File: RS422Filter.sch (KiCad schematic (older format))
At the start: 13 parts, among them J12 Conn_01x02

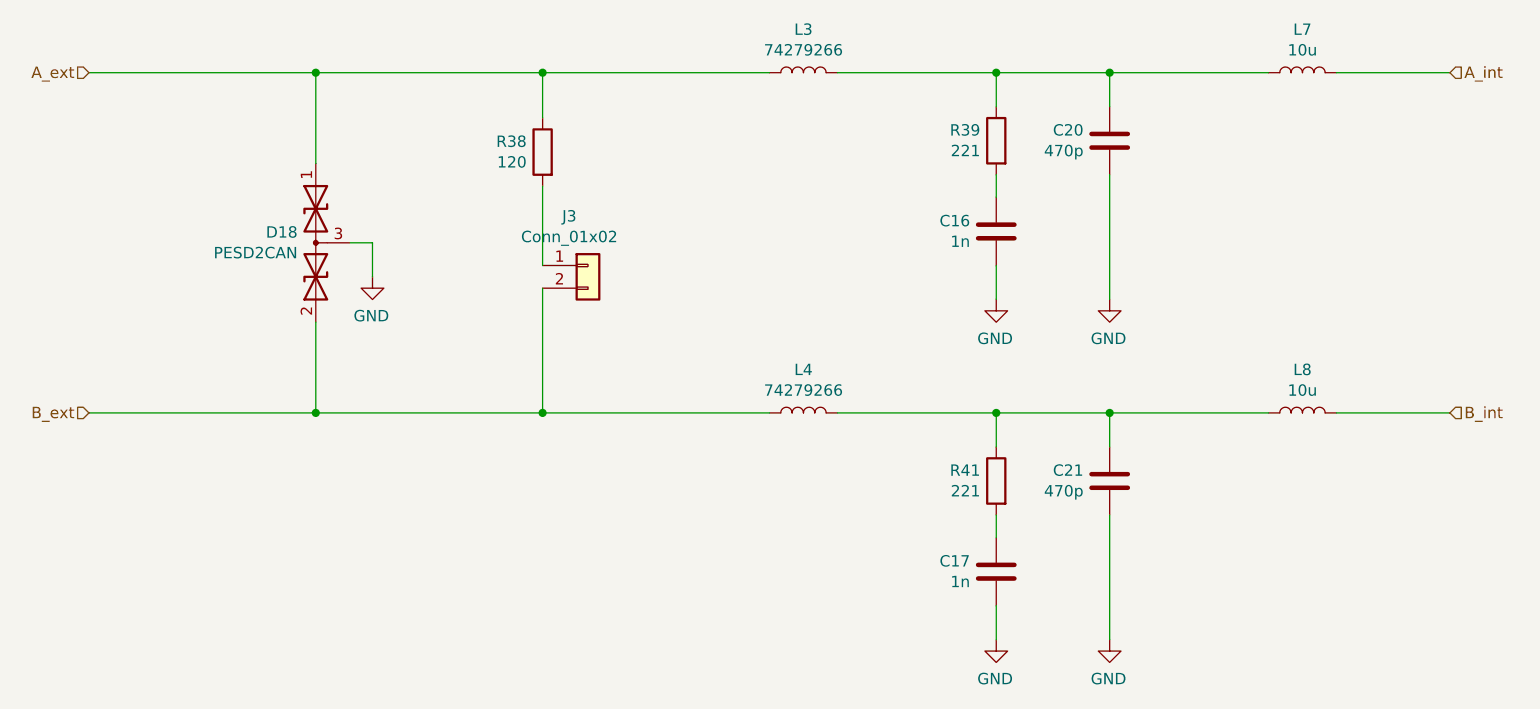
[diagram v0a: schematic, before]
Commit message: routing
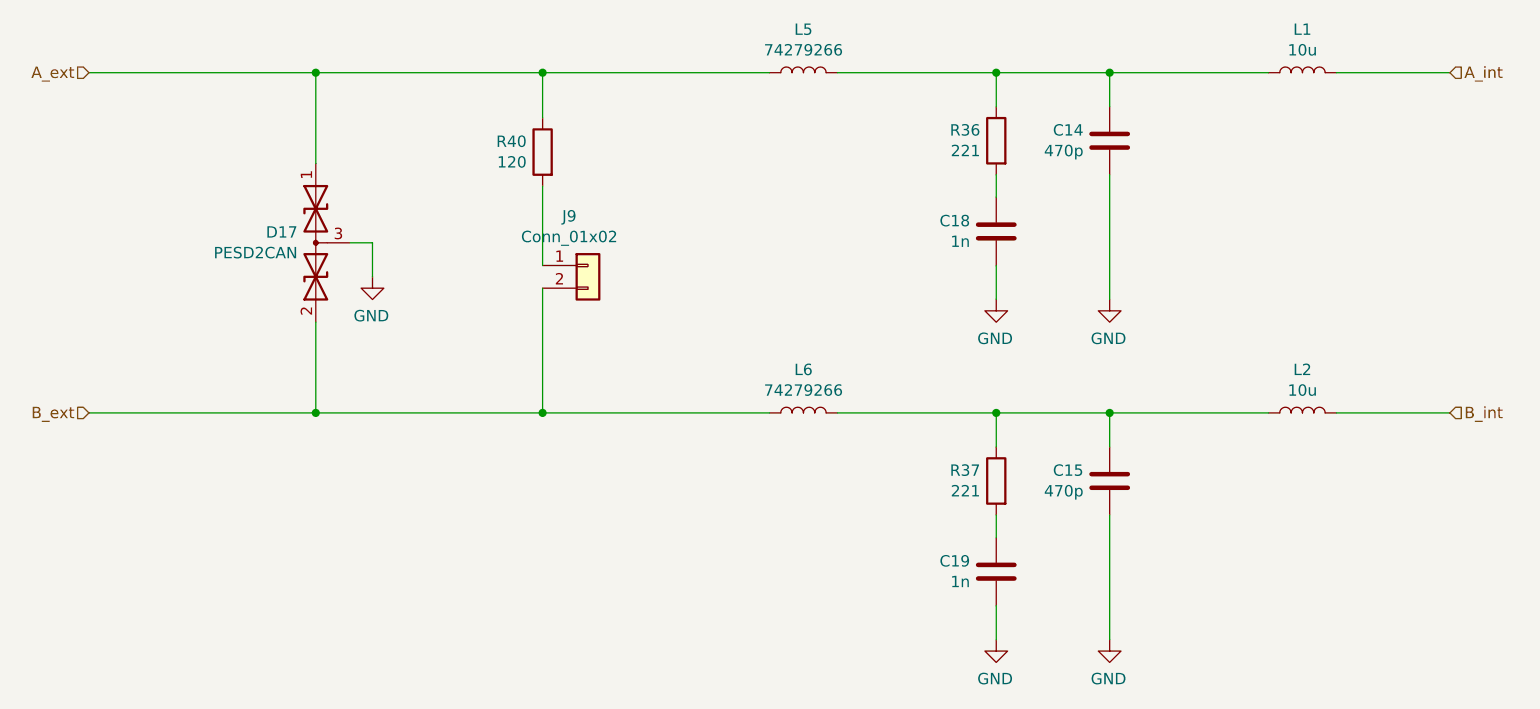
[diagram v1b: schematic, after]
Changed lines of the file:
@@
 $Descr A4 11693 8268
 encoding utf-8
-Sheet 5 22
+Sheet 4 22
 Title ""
 Date ""
@@
 AR Path="/6089ADE2/608D0C52/608D8603" Ref="D?"  Part="1"
 AR Path="/6089ADE2/608DD62D/608D8603" Ref="D18"  Part="1"
-F 0 "D18" V 3404 3330 50  0000 L CNN
+F 0 "D17" V 3404 3330 50  0000 L CNN
 F 1 "PESD2CAN" V 3495 3330 50  0000 L CNN
 F 2 "Package_TO_SOT_SMD:SOT-23_Handsoldering" H 3300 3250 50  0001 C CNN
@@
 AR Path="/6089ADE2/608D0C52/608D8609" Ref="L?"  Part="1"
 AR Path="/6089ADE2/608DD62D/608D8609" Ref="L3"  Part="1"
-F 0 "L3" V 5790 2500 50  0000 C CNN
+F 0 "L5" V 5790 2500 50  0000 C CNN
 F 1 "74279266" V 5699 2500 50  0000 C CNN
 F 2 "Inductor_SMD:L_0603_1608Metric" H 5600 2500 50  0001 C CNN
@@
 AR Path="/6089ADE2/608D0C52/608D985F" Ref="R?"  Part="1"
 AR Path="/6089ADE2/608DD62D/608D985F" Ref="R39"  Part="1"
-F 0 "R39" H 6520 2846 50  0000 L CNN
+F 0 "R36" H 6520 2846 50  0000 L CNN
 F 1 "221" H 6520 2755 50  0000 L CNN
 F 2 "Resistor_SMD:R_0603_1608Metric" V 6380 2800 50  0001 C CNN
@@
 AR Path="/6089ADE2/608D0C52/608D9BE8" Ref="C?"  Part="1"
 AR Path="/6089ADE2/608DD62D/608D9BE8" Ref="C16"  Part="1"
-F 0 "C16" H 6565 3246 50  0000 L CNN
+F 0 "C18" H 6565 3246 50  0000 L CNN
 F 1 "1n" H 6565 3155 50  0000 L CNN
 F 2 "Capacitor_SMD:C_0603_1608Metric" H 6488 3050 50  0001 C CNN
@@
 AR Path="/6089ADE2/608D0C52/608DA048" Ref="C?"  Part="1"
 AR Path="/6089ADE2/608DD62D/608DA048" Ref="C20"  Part="1"
-F 0 "C20" H 7065 2846 50  0000 L CNN
+F 0 "C14" H 7065 2846 50  0000 L CNN
 F 1 "470p" H 7065 2755 50  0000 L CNN
 F 2 "Capacitor_SMD:C_0603_1608Metric" H 6988 2650 50  0001 C CNN
@@
 AR Path="/6089ADE2/608D0C52/608DA55F" Ref="L?"  Part="1"
 AR Path="/6089ADE2/608DD62D/608DA55F" Ref="L7"  Part="1"
-F 0 "L7" V 7990 2500 50  0000 C CNN
+F 0 "L1" V 7990 2500 50  0000 C CNN
 F 1 "10u" V 7899 2500 50  0000 C CNN
 F 2 "Inductor_SMD:L_0603_1608Metric" H 7800 2500 50  0001 C CNN
@@
 AR Path="/6089ADE2/608D0C52/608DBE73" Ref="#PWR?"  Part="1"
 AR Path="/6089ADE2/608DD62D/608DBE73" Ref="#PWR0203"  Part="1"
-F 0 "#PWR0203" H 6450 3250 50  0001 C CNN
+F 0 "#PWR047" H 6450 3250 50  0001 C CNN
 F 1 "GND" H 6455 3327 50  0000 C CNN
 F 2 "" H 6450 3500 50  0001 C CNN
@@
 AR Path="/6089ADE2/608D0C52/608DC4B4" Ref="#PWR?"  Part="1"
 AR Path="/6089ADE2/608DD62D/608DC4B4" Ref="#PWR0204"  Part="1"
-F 0 "#PWR0204" H 6950 3250 50  0001 C CNN
+F 0 "#PWR043" H 6950 3250 50  0001 C CNN
 F 1 "GND" H 6955 3327 50  0000 C CNN
 F 2 "" H 6950 3500 50  0001 C CNN
@@
 AR Path="/6089ADE2/608D0C52/608E2FA4" Ref="L?"  Part="1"
 AR Path="/6089ADE2/608DD62D/608E2FA4" Ref="L4"  Part="1"
-F 0 "L4" V 5790 4000 50  0000 C CNN
+F 0 "L6" V 5790 4000 50  0000 C CNN
 F 1 "74279266" V 5699 4000 50  0000 C CNN
 F 2 "Inductor_SMD:L_0603_1608Metric" H 5600 4000 50  0001 C CNN
@@
 AR Path="/6089ADE2/608D0C52/608E2FAA" Ref="R?"  Part="1"
 AR Path="/6089ADE2/608DD62D/608E2FAA" Ref="R41"  Part="1"
-F 0 "R41" H 6520 4346 50  0000 L CNN
+F 0 "R37" H 6520 4346 50  0000 L CNN
 F 1 "221" H 6520 4255 50  0000 L CNN
 F 2 "Resistor_SMD:R_0603_1608Metric" V 6380 4300 50  0001 C CNN
@@
 AR Path="/6089ADE2/608D0C52/608E2FB0" Ref="C?"  Part="1"
 AR Path="/6089ADE2/608DD62D/608E2FB0" Ref="C17"  Part="1"
-F 0 "C17" H 6565 4746 50  0000 L CNN
+F 0 "C19" H 6565 4746 50  0000 L CNN
 F 1 "1n" H 6565 4655 50  0000 L CNN
 F 2 "Capacitor_SMD:C_0603_1608Metric" H 6488 4550 50  0001 C CNN
@@
 AR Path="/6089ADE2/608D0C52/608E2FB6" Ref="C?"  Part="1"
 AR Path="/6089ADE2/608DD62D/608E2FB6" Ref="C21"  Part="1"
-F 0 "C21" H 7065 4346 50  0000 L CNN
+F 0 "C15" H 7065 4346 50  0000 L CNN
 F 1 "470p" H 7065 4255 50  0000 L CNN
 F 2 "Capacitor_SMD:C_0603_1608Metric" H 6988 4150 50  0001 C CNN
@@
 AR Path="/6089ADE2/608D0C52/608E2FBC" Ref="L?"  Part="1"
 AR Path="/6089ADE2/608DD62D/608E2FBC" Ref="L8"  Part="1"
-F 0 "L8" V 7990 4000 50  0000 C CNN
+F 0 "L2" V 7990 4000 50  0000 C CNN
 F 1 "10u" V 7899 4000 50  0000 C CNN
 F 2 "Inductor_SMD:L_0603_1608Metric" H 7800 4000 50  0001 C CNN
@@
 AR Path="/6089ADE2/608D0C52/608E2FC6" Ref="#PWR?"  Part="1"
 AR Path="/6089ADE2/608DD62D/608E2FC6" Ref="#PWR0205"  Part="1"
-F 0 "#PWR0205" H 6450 4750 50  0001 C CNN
+F 0 "#PWR048" H 6450 4750 50  0001 C CNN
 F 1 "GND" H 6455 4827 50  0000 C CNN
 F 2 "" H 6450 5000 50  0001 C CNN
@@
 AR Path="/6089ADE2/608D0C52/608E2FCD" Ref="#PWR?"  Part="1"
 AR Path="/6089ADE2/608DD62D/608E2FCD" Ref="#PWR0206"  Part="1"
-F 0 "#PWR0206" H 6950 4750 50  0001 C CNN
+F 0 "#PWR044" H 6950 4750 50  0001 C CNN
 F 1 "GND" H 6955 4827 50  0000 C CNN
 F 2 "" H 6950 5000 50  0001 C CNN
@@
 AR Path="/6089ADE2/608D0C52/608E4369" Ref="#PWR?"  Part="1"
 AR Path="/6089ADE2/608DD62D/608E4369" Ref="#PWR0207"  Part="1"
-F 0 "#PWR0207" H 3700 3150 50  0001 C CNN
+F 0 "#PWR051" H 3700 3150 50  0001 C CNN
 F 1 "GND" H 3705 3227 50  0000 C CNN
 F 2 "" H 3700 3400 50  0001 C CNN
@@
 AR Path="/6089ADE2/608D0C52/609E589E" Ref="R?"  Part="1"
 AR Path="/6089ADE2/608DD62D/609E589E" Ref="R38"  Part="1"
-F 0 "R38" H 4520 2896 50  0000 L CNN
+F 0 "R40" H 4520 2896 50  0000 L CNN
 F 1 "120" H 4520 2805 50  0000 L CNN
 F 2 "Resistor_SMD:R_0603_1608Metric" V 4380 2850 50  0001 C CNN
@@
 AR Path="/6089ADE2/608D0C52/609E64E5" Ref="J?"  Part="1"
 AR Path="/6089ADE2/608DD62D/609E64E5" Ref="J3"  Part="1"
-F 0 "J3" H 4568 3567 50  0000 C CNN
+F 0 "J9" H 4568 3567 50  0000 C CNN
 F 1 "Conn_01x02" H 4568 3476 50  0000 C CNN
 F 2 "Connector_PinHeader_2.54mm:PinHeader_1x02_P2.54mm_Vertical" H 4650 3350 50  0001 C CNN

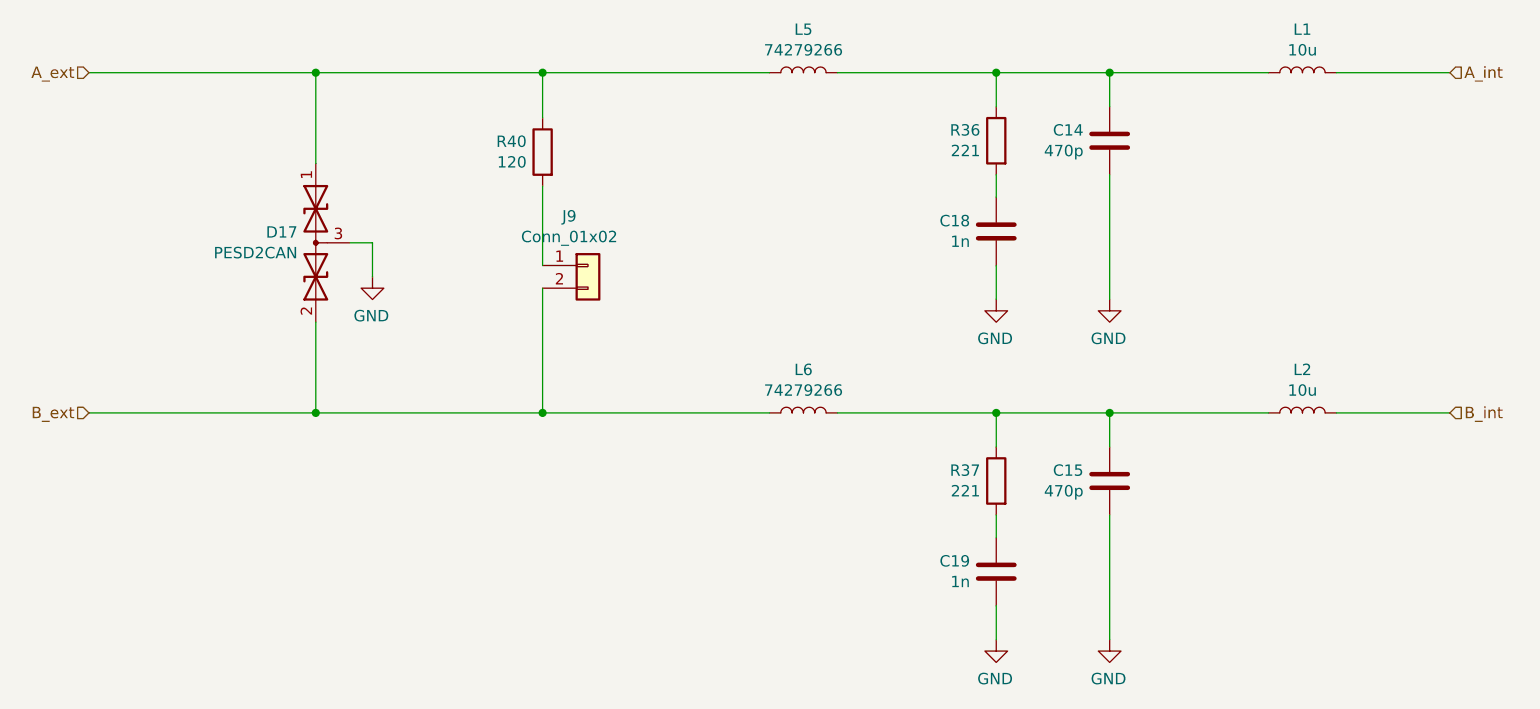
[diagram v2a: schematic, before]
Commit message: placement, routing
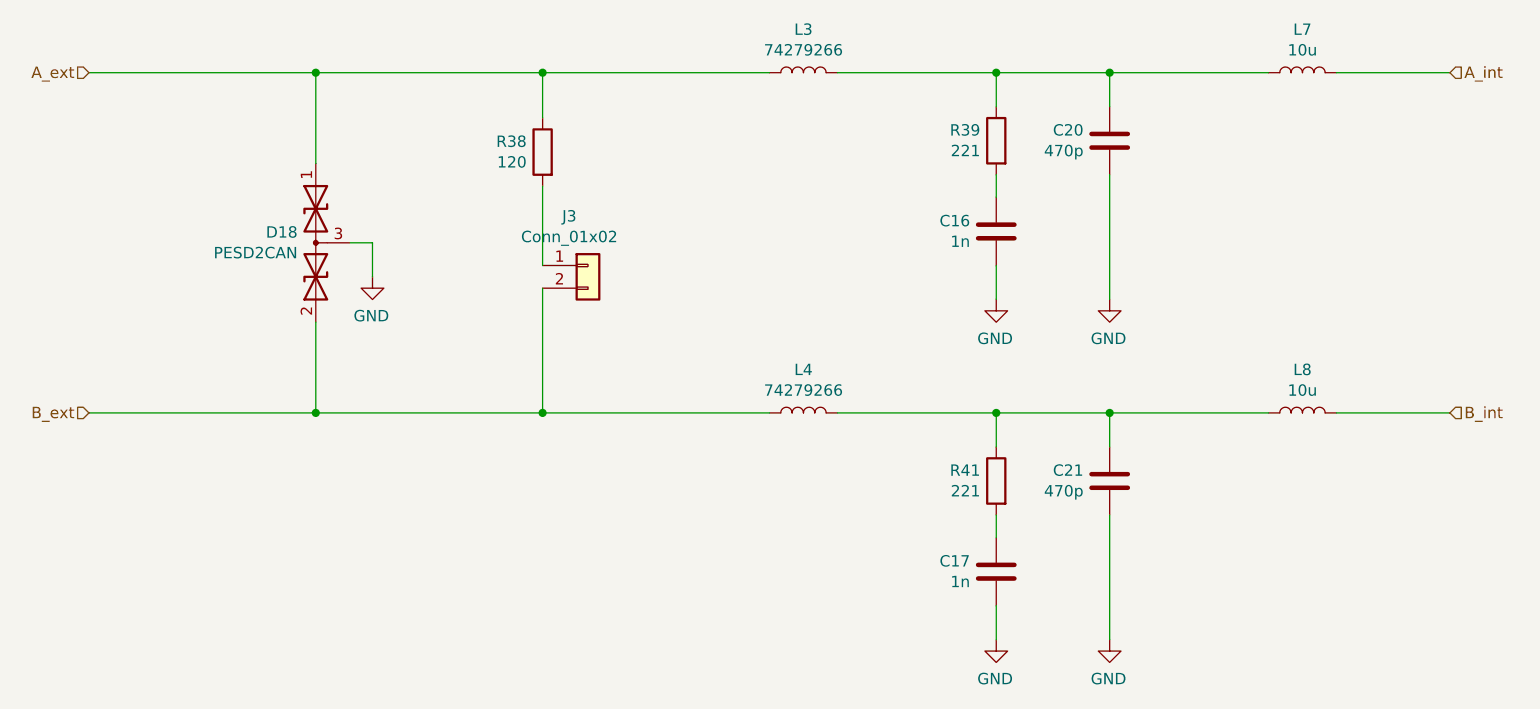
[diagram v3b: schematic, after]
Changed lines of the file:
@@
 $Descr A4 11693 8268
 encoding utf-8
-Sheet 4 22
+Sheet 5 22
 Title ""
 Date ""
@@
 AR Path="/6089ADE2/608D0C52/608D8603" Ref="D?"  Part="1"
 AR Path="/6089ADE2/608DD62D/608D8603" Ref="D18"  Part="1"
-F 0 "D17" V 3404 3330 50  0000 L CNN
+F 0 "D18" V 3404 3330 50  0000 L CNN
 F 1 "PESD2CAN" V 3495 3330 50  0000 L CNN
 F 2 "Package_TO_SOT_SMD:SOT-23_Handsoldering" H 3300 3250 50  0001 C CNN
@@
 AR Path="/6089ADE2/608D0C52/608D8609" Ref="L?"  Part="1"
 AR Path="/6089ADE2/608DD62D/608D8609" Ref="L3"  Part="1"
-F 0 "L5" V 5790 2500 50  0000 C CNN
+F 0 "L3" V 5790 2500 50  0000 C CNN
 F 1 "74279266" V 5699 2500 50  0000 C CNN
 F 2 "Inductor_SMD:L_0603_1608Metric" H 5600 2500 50  0001 C CNN
@@
 AR Path="/6089ADE2/608D0C52/608D985F" Ref="R?"  Part="1"
 AR Path="/6089ADE2/608DD62D/608D985F" Ref="R39"  Part="1"
-F 0 "R36" H 6520 2846 50  0000 L CNN
+F 0 "R39" H 6520 2846 50  0000 L CNN
 F 1 "221" H 6520 2755 50  0000 L CNN
 F 2 "Resistor_SMD:R_0603_1608Metric" V 6380 2800 50  0001 C CNN
@@
 AR Path="/6089ADE2/608D0C52/608D9BE8" Ref="C?"  Part="1"
 AR Path="/6089ADE2/608DD62D/608D9BE8" Ref="C16"  Part="1"
-F 0 "C18" H 6565 3246 50  0000 L CNN
+F 0 "C16" H 6565 3246 50  0000 L CNN
 F 1 "1n" H 6565 3155 50  0000 L CNN
 F 2 "Capacitor_SMD:C_0603_1608Metric" H 6488 3050 50  0001 C CNN
@@
 AR Path="/6089ADE2/608D0C52/608DA048" Ref="C?"  Part="1"
 AR Path="/6089ADE2/608DD62D/608DA048" Ref="C20"  Part="1"
-F 0 "C14" H 7065 2846 50  0000 L CNN
+F 0 "C20" H 7065 2846 50  0000 L CNN
 F 1 "470p" H 7065 2755 50  0000 L CNN
 F 2 "Capacitor_SMD:C_0603_1608Metric" H 6988 2650 50  0001 C CNN
@@
 AR Path="/6089ADE2/608D0C52/608DA55F" Ref="L?"  Part="1"
 AR Path="/6089ADE2/608DD62D/608DA55F" Ref="L7"  Part="1"
-F 0 "L1" V 7990 2500 50  0000 C CNN
+F 0 "L7" V 7990 2500 50  0000 C CNN
 F 1 "10u" V 7899 2500 50  0000 C CNN
 F 2 "Inductor_SMD:L_0603_1608Metric" H 7800 2500 50  0001 C CNN
@@
 AR Path="/6089ADE2/608D0C52/608E2FA4" Ref="L?"  Part="1"
 AR Path="/6089ADE2/608DD62D/608E2FA4" Ref="L4"  Part="1"
-F 0 "L6" V 5790 4000 50  0000 C CNN
+F 0 "L4" V 5790 4000 50  0000 C CNN
 F 1 "74279266" V 5699 4000 50  0000 C CNN
 F 2 "Inductor_SMD:L_0603_1608Metric" H 5600 4000 50  0001 C CNN
@@
 AR Path="/6089ADE2/608D0C52/608E2FAA" Ref="R?"  Part="1"
 AR Path="/6089ADE2/608DD62D/608E2FAA" Ref="R41"  Part="1"
-F 0 "R37" H 6520 4346 50  0000 L CNN
+F 0 "R41" H 6520 4346 50  0000 L CNN
 F 1 "221" H 6520 4255 50  0000 L CNN
 F 2 "Resistor_SMD:R_0603_1608Metric" V 6380 4300 50  0001 C CNN
@@
 AR Path="/6089ADE2/608D0C52/608E2FB0" Ref="C?"  Part="1"
 AR Path="/6089ADE2/608DD62D/608E2FB0" Ref="C17"  Part="1"
-F 0 "C19" H 6565 4746 50  0000 L CNN
+F 0 "C17" H 6565 4746 50  0000 L CNN
 F 1 "1n" H 6565 4655 50  0000 L CNN
 F 2 "Capacitor_SMD:C_0603_1608Metric" H 6488 4550 50  0001 C CNN
@@
 AR Path="/6089ADE2/608D0C52/608E2FB6" Ref="C?"  Part="1"
 AR Path="/6089ADE2/608DD62D/608E2FB6" Ref="C21"  Part="1"
-F 0 "C15" H 7065 4346 50  0000 L CNN
+F 0 "C21" H 7065 4346 50  0000 L CNN
 F 1 "470p" H 7065 4255 50  0000 L CNN
 F 2 "Capacitor_SMD:C_0603_1608Metric" H 6988 4150 50  0001 C CNN
@@
 AR Path="/6089ADE2/608D0C52/608E2FBC" Ref="L?"  Part="1"
 AR Path="/6089ADE2/608DD62D/608E2FBC" Ref="L8"  Part="1"
-F 0 "L2" V 7990 4000 50  0000 C CNN
+F 0 "L8" V 7990 4000 50  0000 C CNN
 F 1 "10u" V 7899 4000 50  0000 C CNN
 F 2 "Inductor_SMD:L_0603_1608Metric" H 7800 4000 50  0001 C CNN
@@
 AR Path="/6089ADE2/608D0C52/609E589E" Ref="R?"  Part="1"
 AR Path="/6089ADE2/608DD62D/609E589E" Ref="R38"  Part="1"
-F 0 "R40" H 4520 2896 50  0000 L CNN
+F 0 "R38" H 4520 2896 50  0000 L CNN
 F 1 "120" H 4520 2805 50  0000 L CNN
 F 2 "Resistor_SMD:R_0603_1608Metric" V 4380 2850 50  0001 C CNN
@@
 AR Path="/6089ADE2/608D0C52/609E64E5" Ref="J?"  Part="1"
 AR Path="/6089ADE2/608DD62D/609E64E5" Ref="J3"  Part="1"
-F 0 "J9" H 4568 3567 50  0000 C CNN
+F 0 "J3" H 4568 3567 50  0000 C CNN
 F 1 "Conn_01x02" H 4568 3476 50  0000 C CNN
 F 2 "Connector_PinHeader_2.54mm:PinHeader_1x02_P2.54mm_Vertical" H 4650 3350 50  0001 C CNN
